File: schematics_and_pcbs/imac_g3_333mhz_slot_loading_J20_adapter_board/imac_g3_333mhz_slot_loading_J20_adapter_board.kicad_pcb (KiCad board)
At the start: 2 copper layers, 82.5 x 52.5 mm, 21 parts, among them J1 Screw_Terminal_01x06, J2 Conn_02x10_Odd_Even, J3 Conn_02x03_Odd_Even, J4 DB15_Female_HighDensity, J5 Conn_02x03_Odd_Even, U1 ATmega328-PU, U2 LCC110, Y1 Crystal

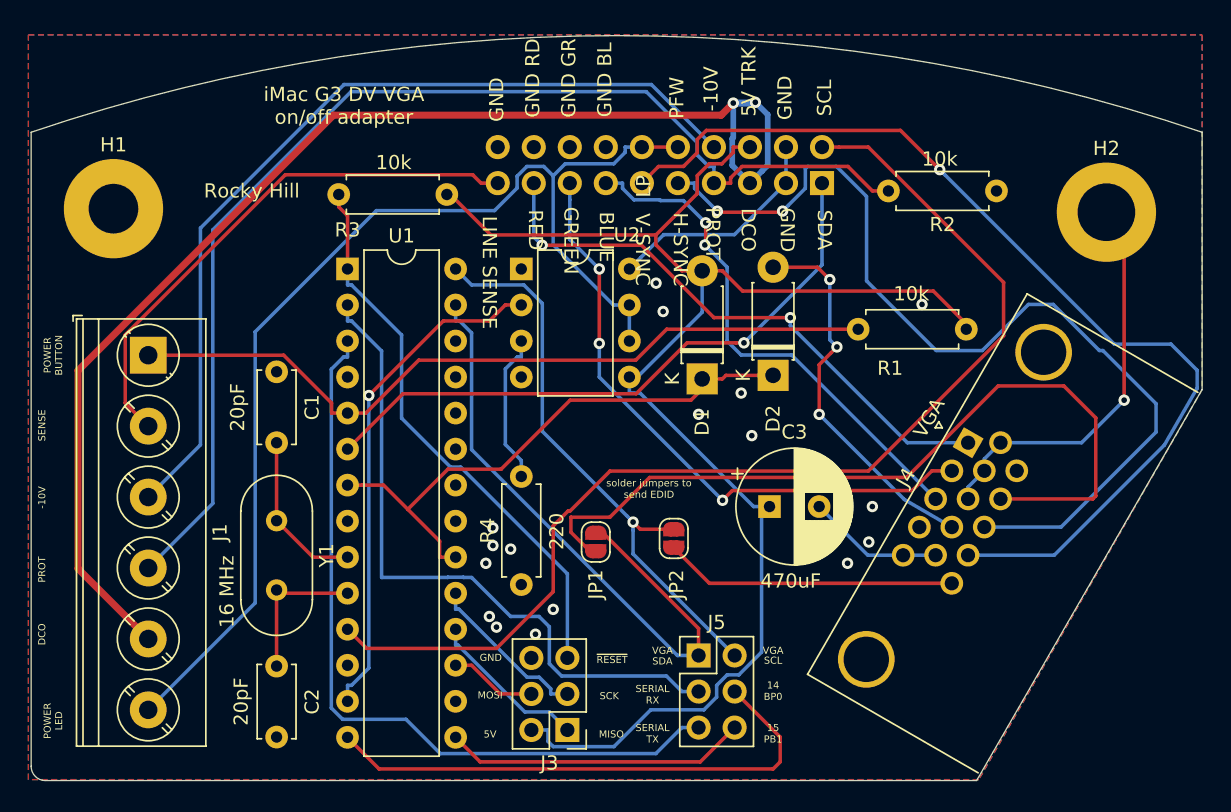
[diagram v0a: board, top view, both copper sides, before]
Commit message: updated silkscreen to make it more readable
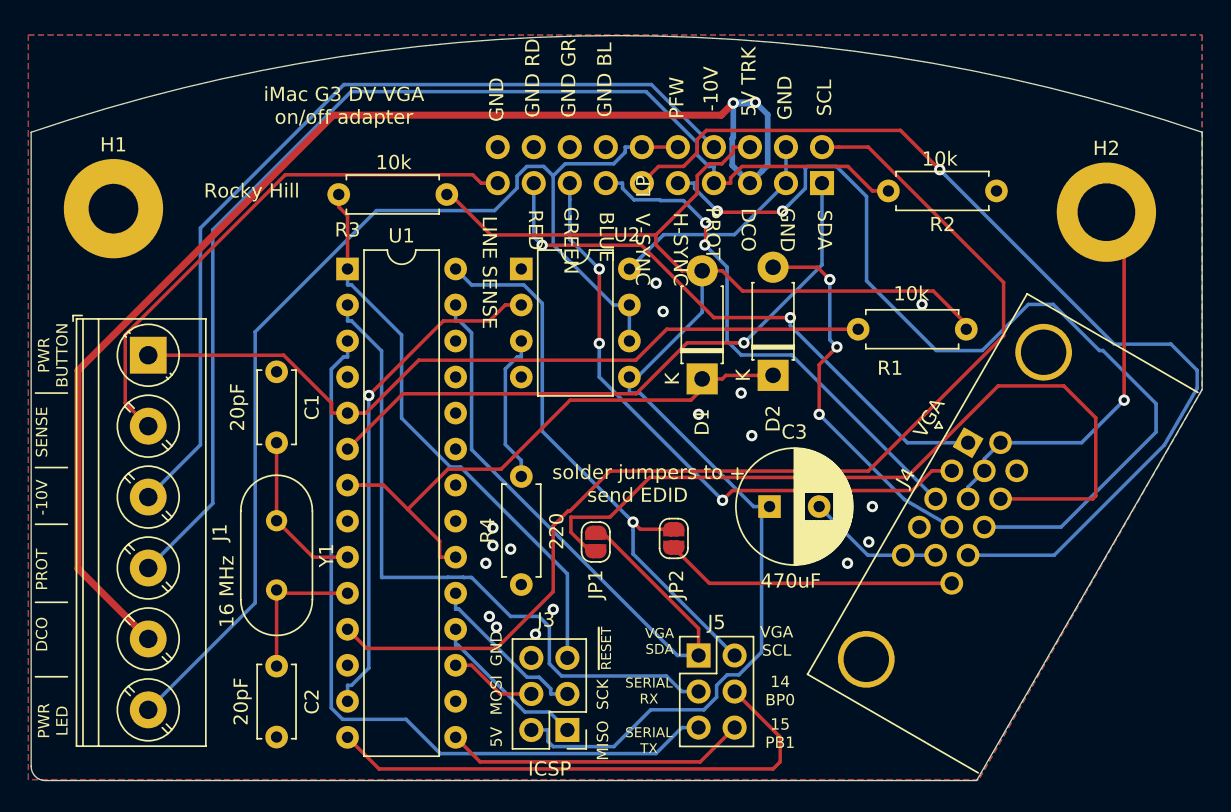
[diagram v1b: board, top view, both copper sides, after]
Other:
- board text added: "ICSP"
- board text added: "PWR BUTTON"
- board text added: "PWR LED"
- board text added: "VGA SCL"
- board text added: "VGA SDA"
- board text removed: "POWER BUTTON"
- board text removed: "POWER LED"
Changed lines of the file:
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@@
   (general
     (thickness 1.6)
-    (drawings 59)
+    (drawings 63)
     (tracks 401)
     (zones 0)
@@
     (31 B.Cu signal)
     (32 B.Adhes user)
-    (33 F.Adhes user hide)
+    (33 F.Adhes user)
     (34 B.Paste user)
     (35 F.Paste user)
@@
     (descr "Through hole straight pin header, 2x03, 2.54mm pitch, double rows")
     (tags "Through hole pin header THT 2x03 2.54mm double row")
-    (fp_text reference J3 (at 1.27 -2.33) (layer F.SilkS)
+    (fp_text reference J3 (at 1.5 7.7502) (layer F.SilkS)
       (effects (font (size 1 1) (thickness 0.15)))
     )
@@
     )
   )
+  (gr_line (start 135.903 82.9038) (end 133.653 82.9038) (layer F.SilkS) (width 0.12))
+  (gr_line (start 135.903 88.1538) (end 133.653 88.1538) (layer F.SilkS) (width 0.12))
+  (gr_line (start 135.903 92.1538) (end 133.653 92.1538) (layer F.SilkS) (width 0.12))
+  (gr_line (start 135.903 97.6538) (end 133.653 97.6538) (layer F.SilkS) (width 0.12))
+  (gr_line (start 135.903 102.9038) (end 133.653 102.9038) (layer F.SilkS) (width 0.12))
+  (gr_text ICSP (at 169.903 109.4038) (layer F.SilkS)
+    (effects (font (size 1 1) (thickness 0.15)))
+  )
   (gr_text "Yeah, cute. Don't get too attached there, \nAladdin, 'cause it's about to be magic flying dinner." (at 159.153 86.4038 90) (layer B.SilkS)
     (effects (font (size 1 1) (thickness 0.15)) (justify mirror))
@@
     (effects (font (size 1 1) (thickness 0.15)))
   )
-  (gr_text VGA (at 185.653 101.0538) (layer F.SilkS)
-    (effects (font (size 0.5 0.5) (thickness 0.1)))
-  )
-  (gr_text VGA (at 177.853 101.0538) (layer F.SilkS)
-    (effects (font (size 0.5 0.5) (thickness 0.1)))
-  )
-  (gr_text "14\nBP0" (at 185.653 103.9038) (layer F.SilkS)
-    (effects (font (size 0.5 0.5) (thickness 0.1)))
-  )
-  (gr_text "15\nPB1" (at 185.653 106.9038) (layer F.SilkS)
-    (effects (font (size 0.5 0.5) (thickness 0.1)))
-  )
-  (gr_text SCL (at 185.653 101.7538) (layer F.SilkS)
-    (effects (font (size 0.5 0.5) (thickness 0.1)))
-  )
-  (gr_text "SERIAL\nTX" (at 177.153 106.9038) (layer F.SilkS)
-    (effects (font (size 0.5 0.5) (thickness 0.1)))
-  )
-  (gr_text SDA (at 177.853 101.8038) (layer F.SilkS)
-    (effects (font (size 0.5 0.5) (thickness 0.1)))
-  )
-  (gr_text "SERIAL\nRX" (at 177.153 104.1538) (layer F.SilkS)
-    (effects (font (size 0.5 0.5) (thickness 0.1)))
-  )
-  (gr_text 5V (at 165.703 106.9538) (layer F.SilkS)
-    (effects (font (size 0.5 0.5) (thickness 0.1)))
-  )
-  (gr_text MOSI (at 165.703 104.2038) (layer F.SilkS)
-    (effects (font (size 0.5 0.5) (thickness 0.1)))
-  )
-  (gr_text GND (at 165.753 101.5538) (layer F.SilkS)
-    (effects (font (size 0.5 0.5) (thickness 0.1)))
-  )
-  (gr_text MISO (at 174.253 106.9538) (layer F.SilkS)
-    (effects (font (size 0.5 0.5) (thickness 0.1)))
-  )
-  (gr_text SCK (at 174.103 104.2538) (layer F.SilkS)
-    (effects (font (size 0.5 0.5) (thickness 0.1)))
-  )
-  (gr_text ~RESET (at 174.303 101.7038) (layer F.SilkS)
-    (effects (font (size 0.5 0.5) (thickness 0.1)))
+  (gr_text "VGA\nSCL" (at 185.903 100.4038) (layer F.SilkS)
+    (effects (font (size 0.8 0.8) (thickness 0.15)))
+  )
+  (gr_text "VGA\nSDA" (at 177.653 100.4038) (layer F.SilkS)
+    (effects (font (size 0.7 0.7) (thickness 0.15)))
+  )
+  (gr_text "14\nBP0" (at 186.153 103.9038) (layer F.SilkS)
+    (effects (font (size 0.8 0.8) (thickness 0.15)))
+  )
+  (gr_text "15\nPB1" (at 186.153 106.9038) (layer F.SilkS)
+    (effects (font (size 0.8 0.8) (thickness 0.15)))
+  )
+  (gr_text "SERIAL\nTX" (at 176.903 107.4038) (layer F.SilkS)
+    (effects (font (size 0.7 0.7) (thickness 0.15)))
+  )
+  (gr_text "SERIAL\nRX" (at 176.903 103.9038) (layer F.SilkS)
+    (effects (font (size 0.7 0.7) (thickness 0.15)))
+  )
+  (gr_text 5V (at 166.153 107.1538 90) (layer F.SilkS)
+    (effects (font (size 0.8 0.8) (thickness 0.15)))
+  )
+  (gr_text MOSI (at 166.153 104.2038 90) (layer F.SilkS)
+    (effects (font (size 0.8 0.8) (thickness 0.15)))
+  )
+  (gr_text GND (at 166.153 100.9038 90) (layer F.SilkS)
+    (effects (font (size 0.8 0.8) (thickness 0.15)))
+  )
+  (gr_text MISO (at 173.653 107.4038 90) (layer F.SilkS)
+    (effects (font (size 0.8 0.8) (thickness 0.15)))
+  )
+  (gr_text SCK (at 173.653 104.1538 90) (layer F.SilkS)
+    (effects (font (size 0.8 0.8) (thickness 0.15)))
+  )
+  (gr_text ~RESET (at 173.903 100.9038 90) (layer F.SilkS)
+    (effects (font (size 0.7 0.7) (thickness 0.15)))
   )
   (gr_line (start 200.003 110.22) (end 134.35 110.22) (layer Edge.Cuts) (width 0.05))
@@
     (effects (font (size 1 1) (thickness 0.15)))
   )
-  (gr_text "solder jumpers to\nsend EDID" (at 176.903 89.6538) (layer F.SilkS)
-    (effects (font (size 0.5 0.5) (thickness 0.1)))
+  (gr_text "solder jumpers to\nsend EDID" (at 176.103 89.3038) (layer F.SilkS)
+    (effects (font (size 1 1) (thickness 0.15)))
   )
   (gr_line (start 133.35 109.22) (end 133.35 64.516001) (layer Edge.Cuts) (width 0.05))
-  (gr_text "POWER\nLED" (at 134.9 106.012 90) (layer F.SilkS)
-    (effects (font (size 0.5 0.5) (thickness 0.1)))
-  )
-  (gr_text "POWER\nBUTTON" (at 134.9 80.236 90) (layer F.SilkS)
-    (effects (font (size 0.5 0.5) (thickness 0.1)))
-  )
-  (gr_text SENSE (at 134.112 85.184 90) (layer F.SilkS)
-    (effects (font (size 0.5 0.5) (thickness 0.1)))
+  (gr_text "PWR\nLED" (at 134.9 106.012 90) (layer F.SilkS)
+    (effects (font (size 0.8 0.8) (thickness 0.15)))
+  )
+  (gr_text "PWR\nBUTTON" (at 134.9 80.236 90) (layer F.SilkS)
+    (effects (font (size 0.8 0.8) (thickness 0.15)))
+  )
+  (gr_text SENSE (at 134.112 85.6538 90) (layer F.SilkS)
+    (effects (font (size 0.8 0.8) (thickness 0.15)))
   )
   (gr_text DCO (at 134.112 99.916 90) (layer F.SilkS)
-    (effects (font (size 0.5 0.5) (thickness 0.1)))
+    (effects (font (size 0.8 0.8) (thickness 0.15)))
   )
   (gr_text PROT (at 134.112 95.344 90) (layer F.SilkS)
-    (effects (font (size 0.5 0.5) (thickness 0.1)))
+    (effects (font (size 0.8 0.8) (thickness 0.15)))
   )
   (gr_text -10V (at 134.112 90.264 90) (layer F.SilkS)
-    (effects (font (size 0.5 0.5) (thickness 0.1)))
+    (effects (font (size 0.8 0.8) (thickness 0.15)))
   )
   (gr_arc (start 174.625 186.181998) (end 215.899998 64.516) (angle -37.47884973) (layer Edge.Cuts) (width 0.05))
